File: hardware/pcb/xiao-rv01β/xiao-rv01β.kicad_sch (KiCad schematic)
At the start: 74 parts, among them J1 Conn_01x02_Pin, J2 Conn_01x02_Socket, J3 Conn_01x02_Socket, J4 Conn_01x02_Pin, J5 Conn_01x02_Socket, J6 Conn_01x02_Pin, J7 Conn_01x04_Pin, J8 Conn_01x10_Pin, J9 Conn_02x10_Pin, M1 DC_Motor_3V, M2 DC_Motor_3V, Q1 P-Ch -12V/-6A, Q2 P-Ch -12V/-6A, SW1 SW_SPDT, SW2 SW_Push, SW3 SW_Push, SW4 SW_Push, SW5 SW_Push, SW6 SW_Push, U1 XIAO ESP32C6, U2 ADS1015, U3 ADS1015, U4 DRV8835, U5 MCP23017

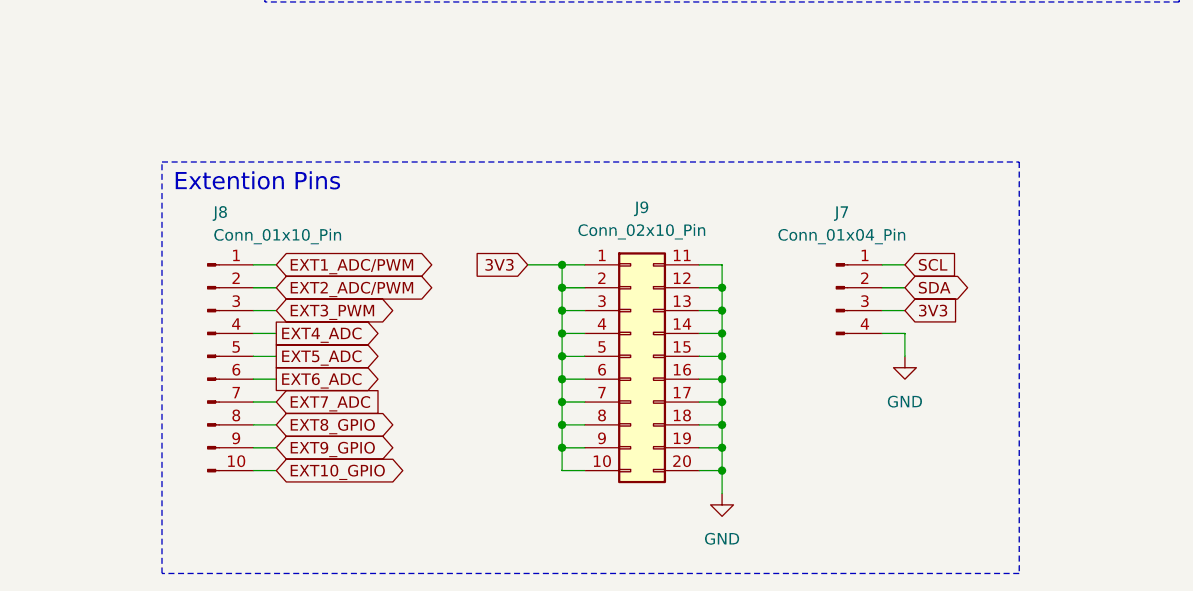
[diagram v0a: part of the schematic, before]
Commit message: initialize PCB
Signed-off-by: Takuto Nagami <logica0419@gmail.com>
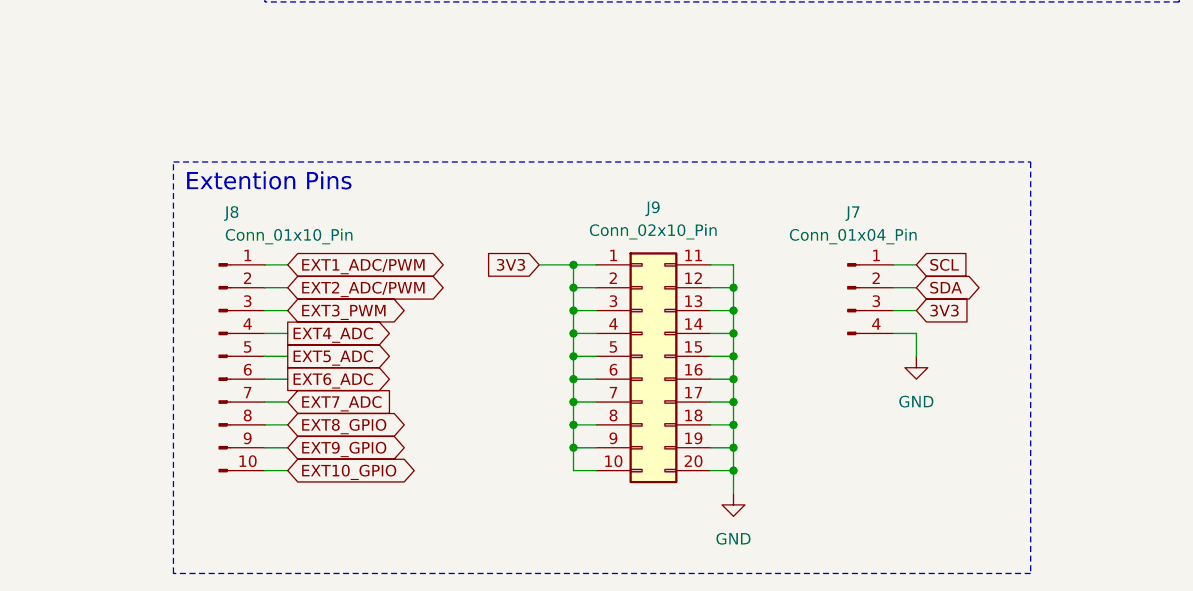
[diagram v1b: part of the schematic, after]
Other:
- moved on the sheet: J7, J8, J9

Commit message: switched to xiao esp32s3 plus & SPI-based expansion
Signed-off-by: Takuto Nagami <logica0419@gmail.com>
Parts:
- removed C10: 47µF/10V, symbol Device:C
- removed C7: 0.1μF, symbol Device:C
- removed J1: Conn_01x02_Pin, symbol Connector:Conn_01x02_Pin
- removed J2: Conn_01x02_Socket, symbol Connector:Conn_01x02_Socket
- removed R11, R12: 4.7kΩ, symbol Device:R
- removed SEN5: GP2Y0E03, symbol GP2Y0E03:GP2Y0E03
- removed U1: XIAO ESP32C6, New_XIAO_Series_Footprints:XIAO-ESP32-C6-DIP, symbol Seeed_Studio_XIAO_Series:XIAO-ESP32-C6-SMD
- removed U2, U3: ADS1015, Package_SO:TSSOP-10_3x3mm_P0.5mm, symbol Analog_ADC:ADS1015IDGS
- removed U5: MCP23017, Package_DIP:DIP-28_W7.62mm, symbol Interface_Expansion:MCP23017x-x-SP
- added C9: 470µF/10V, symbol Device:C
- added J6: Conn_02x05_Top_Bottom, symbol Connector_Generic:Conn_02x05_Top_Bottom
- added R14, R15: 8.2kΩ, symbol Device:R
- added R16, R20: 2.2kΩ, Resistor_THT:R_Axial_DIN0207_L6.3mm_D2.5mm_P7.62mm_Horizontal, symbol Device:R
- added R23: 33kΩ, symbol Device:R
- added R24: 22kΩ, symbol Device:R
- added R8: 22kΩ, Resistor_THT:R_Axial_DIN0207_L6.3mm_D2.5mm_P10.16mm_Horizontal, symbol Device:R
- added SEN5: HC-SR04, symbol HC-SR04:HC-SR04
- added U1: XIAO-ESP32-S3-Plus, New_XIAO_Series_Footprints:XIAO-ESP32-S3-Plus-SMD, symbol Seeed_Studio_XIAO_Series:XIAO-ESP32-S3 Plus-SMD
- added U2: MCP3208, Package_DIP:DIP-16_W7.62mm_Socket, symbol Analog_ADC:MCP3208
- added U4: MCP23S17, Package_DIP:DIP-28_W7.62mm_Socket, symbol Interface_Expansion:MCP23S17x-x-SP
- C4: value 47µF/10V -> 470µF/10V
- J7: renamed from J8; value Conn_01x10_Pin -> Conn_01x12_Pin; symbol Connector:Conn_01x10_Pin -> Connector:Conn_01x12_Pin
- J8: renamed from J9; value Conn_02x10_Pin -> Conn_02x12_Top_Bottom; symbol Connector_Generic:Conn_02x10_Top_Bottom -> Connector_Generic:Conn_02x12_Top_Bottom
- R1: renamed from R5; value 100kΩ -> 33kΩ
- R10: renamed from R7; value 33kΩ -> 100kΩ
- R12: renamed from R10; value 4.7kΩ -> 8.2kΩ
- R13: value 4.7kΩ -> 8.2kΩ
- renumbered C9 to C7, J3 to J1, J4 to J2, J5 to J3, J6 to J4, J7 to J5, LED5 to LED1, LED1 to LED2, LED6 to LED4, LED2 to LED5, LED4 to LED6, R14 to R11, R16 to R18, R15 to R19, R8 to R2, R19 to R21, R18 to R22, R20 to R25, R6 to R3, R1 to R4, R2 to R5, R3 to R6, R4 to R7, U4 to U3
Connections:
- net 3V3: now also J8.11 (Pin_11), J8.12 (Pin_12), R16.1, R20.1, U1.12 (3V3), U2.15 (Vref), U2.16 (Vdd), U4.18 (~{RESET}), U4.9 (V_{DD})
- net BUZZER: now also U1.7 (GPIO43_D6_TX)
- net EXT10_GPIO: now also U4.21 (GPA0)
- net EXT1_ADC/PWM: now also U1.2 (GPIO2_A1_D1)
- net EXT2_ADC/PWM: now also U1.3 (GPIO3_A2_D2)
- net EXT6_ADC: now also U2.5 (CH4)
- net EXT7_ADC: now also U2.6 (CH5)
- net GND: now also J8.21 (Pin_21), J8.22 (Pin_22), J8.23 (Pin_23), J8.24 (Pin_24), C9.1, J6.10 (Pin_10), J6.6 (Pin_6), J6.7 (Pin_7), J6.8 (Pin_8), J6.9 (Pin_9), R14.2, R15.2, R23.1, SEN5.4 (GND), U1.13 (GND), U1.33 (GND2), U1.34 (PAD), U2.14 (AGND), U2.9 (DGND), U4.10 (V_{SS}), U4.15 (A0), U4.16 (A1), U4.17 (A2); no longer J8.11 (Pin_11), J8.12 (Pin_12)
- net MD_AENBL: now also U1.22 (GPIO12_DVP_Y7_SPI_MISO1)
- net MD_APHASE: now also U4.7 (GPB6)
- net MD_BENBL: now also U1.23 (GPIO13_DVP_PCLK_SPI_SCK1)
- net MD_BPHASE: now also U4.8 (GPB7)
- net NEO_PIXEL: now also U1.8 (GPIO44_D7_RX)
- net SCL: now also R16.2, U1.18 (GPIO41_PDM_DATA_RX1); no longer R17.2
- net SDA: now also U1.17 (GPIO40_CAM_SDA_I2S_WS)
- net VBUS: now also R3.2, U1.14 (VBUS); no longer R3.1
- net at SW2.1: now also U4.1 (GPB0)
- net at SW3.1: now also U4.2 (GPB1)
- net at SW4.1: now also U4.3 (GPB2)
- net at SW5.1: now also U4.4 (GPB3)
- net at SW6.1: now also U4.5 (GPB4)
- net at SEN4.4 (E): now also R15.1, U2.1 (CH0); no longer R13.1
- net at SEN3.4 (E): now also R14.1, U2.2 (CH1)
- net at C1.2, R1.2: now also R8.2, U1.1 (GPIO1_A0_D0); no longer R10.1
- net at D1.1 (K), Q1.3 (S), Q2.2 (D)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: now also U1.32 (VBAT)
- net at R11.2, R18.1: now also U1.21 (GPIO11_DVP_Y8_SPI_MOSI1)
- net at Q1.1 (G), R2.1: now also R3.1; no longer R3.2
- net at SEN2.4 (E): now also R13.1, U2.3 (CH2)
- net at R12.1, SEN1.4 (E): now also U2.4 (CH3)
- net EXT3_PWM renamed EXT3_ADC/PWM
- net EXT3_ADC/PWM: now also U1.4 (GPIO4_A3_D3)
- net EXT4_ADC renamed EXT4_ADC/PWM
- net EXT4_ADC/PWM: now also U1.5 (GPIO5_A4_D4_SDA)
- net EXT5_ADC renamed EXT5_ADC/PWM
- net EXT5_ADC/PWM: now also U1.6 (GPIO6_A5_D5_SCL)
- net EXT8_GPIO renamed EXT8_ADC
- net EXT8_ADC: now also U2.7 (CH6)
- net EXT9_GPIO renamed EXT9_ADC
- net EXT9_ADC: now also U2.8 (CH7)
- new net: R10.1, R8.1
- new net: R24.2, SEN5.3 (Echo)
- new net 5V: C9.2, J6.1 (Pin_1), J6.2 (Pin_2), J6.3 (Pin_3), J6.4 (Pin_4), J6.5 (Pin_5), SEN5.1 (Vcc)
- new net ADC_CS: R20.2, U1.20 (GPIO10_XMCLK_ADC_BAT), U2.10 (~{CS}/SHDN)
- new net EXT11_GPIO: J7.11 (Pin_11), U4.22 (GPA1)
- new net EXT12_GPIO: J7.12 (Pin_12), U4.23 (GPA2)
- new net Echo: R23.2, R24.1, U1.16 (GPIO39_CAM_SCL_I2S_SCK)
- new net IOE_CS: R17.2, U1.19 (GPIO42_PDM_CLK_TX1), U4.11 (~{CS})
- new net MISO: U1.10 (GPIO8_A9_D9_MISO), U2.12 (Dout), U4.14 (SO)
- new net MOSI: U1.11 (GPIO9_A10_D10_MOSI), U2.11 (Din), U4.13 (SI)
- new net SCK: U1.9 (GPIO7_A8_D8_SCK), U2.13 (CLK), U4.12 (SCK)
- new net Trigger: SEN5.2 (Trigger), U1.15 (GPIO38_DVP_VSYNC_I2S_SD)
- no-connect marks 21 -> 18
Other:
- note added: "ADC & Reflective Sensors"
- note added: "Extension Pins"
- note removed: "ADC #1 & Reflective Sensors"
- note removed: "ADC #2"
- note removed: "Extention Pins"
- moved on the sheet: BT1, BZ1, C1, C2, C3, C4, C5, C6, C7, D1, F1, FB1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
